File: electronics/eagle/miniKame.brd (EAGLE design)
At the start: 37.8 x 41.9 mm, 17 parts

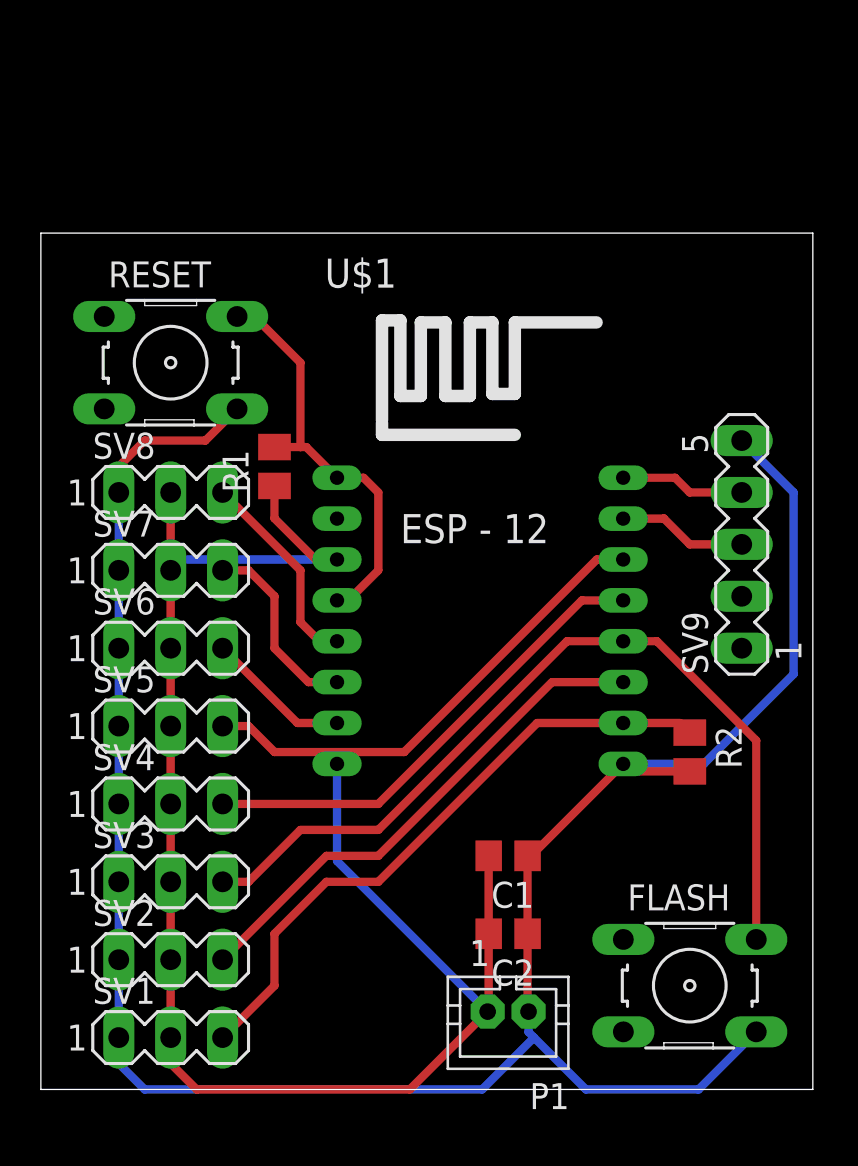
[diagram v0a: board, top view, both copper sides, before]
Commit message: Update pcb
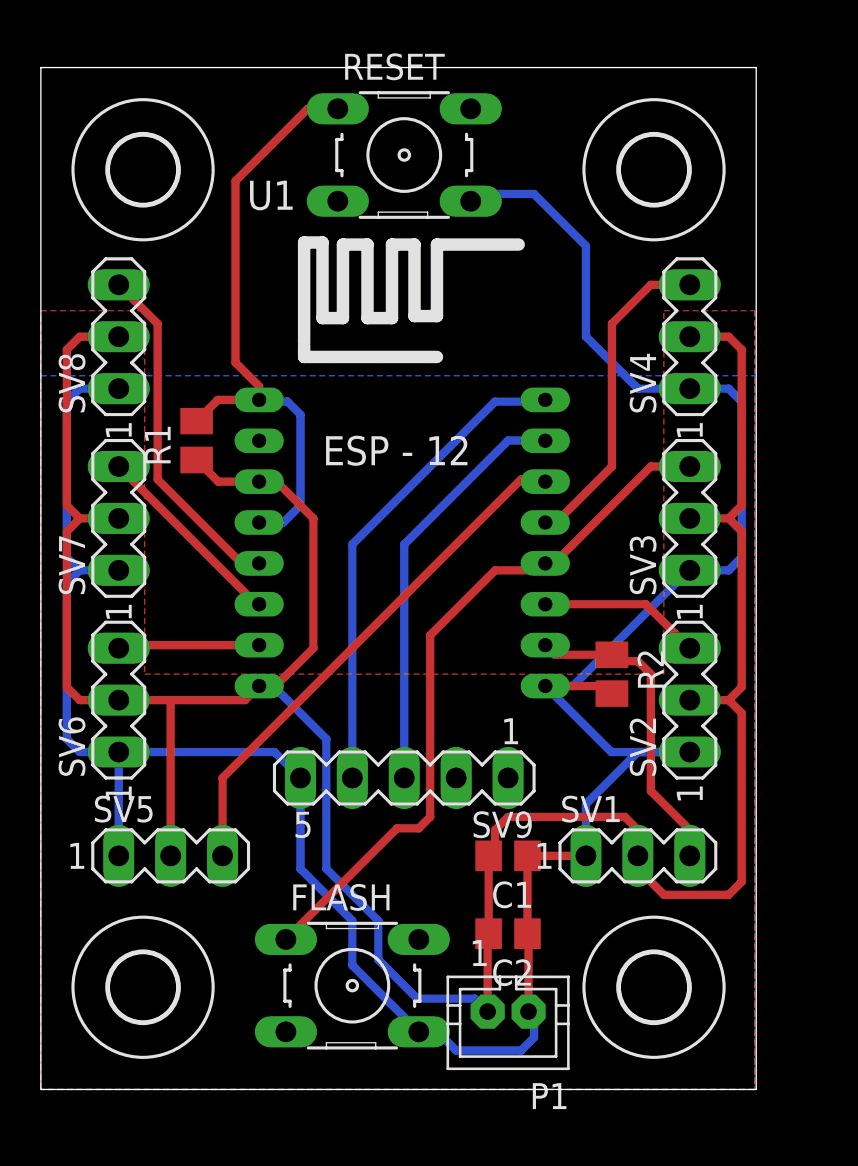
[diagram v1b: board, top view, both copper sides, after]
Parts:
- removed U$1: ESP12, esp8266modules:ESP12
- added H1, H2, H3, H4: MOUNT-HOLE3.3, holes:3,3
- added U1: ESP12, esp8266modules:ESP12
- C1: value (none) -> 100n
- C2: value (none) -> 100u
- moved SV4 34.2 mm to (31.8, 36.8), turned to 90 degrees
- moved SV3 31.0 mm to (31.8, 27.9), turned to 90 degrees
- moved SV2 28.4 mm to (31.8, 19.1), turned to 90 degrees
- moved SV1 24.5 mm to (29.2, 11.4)
- moved SV9 20.1 mm to (17.8, 15.2), turned to 180 degrees
- moved FLASH 16.5 mm to (15.2, 5.08)
- moved RESET 15.3 mm to (17.8, 45.7)
- moved SV8 8.03 mm to (3.81, 36.8), turned to 90 degrees
- moved SV5 6.35 mm to (6.35, 11.4)
- moved R2 5.39 mm to (27.9, 20.3)
- moved R1 4.02 mm to (7.62, 31.8)
- moved SV7 3.59 mm to (3.81, 27.9), turned to 90 degrees
- moved SV6 3.59 mm to (3.81, 19.1), turned to 90 degrees
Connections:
- removed net N$3: SV9.2
- net +3V3: now also U1.CH_PD, U1.VCC; no longer U$1.CH_PD, U$1.VCC
- net GND: now also U1.GND; no longer U$1.GND
- net N$1: now also U1.TX; no longer U$1.TX
- net N$2: now also U1.RX; no longer U$1.RX
- net N$4: now also RESET.1, U1.GPIO16, U1.RESET; no longer RESET.2, U$1.GPIO16, U$1.RESET
- net S1: now also U1.GPIO15; no longer U$1.GPIO15
- net S2: now also U1.GPIO2; no longer U$1.GPIO2
- net S3: now also FLASH.1, U1.GPIO0; no longer FLASH.2, U$1.GPIO0
- net S4: now also U1.GPIO5; no longer U$1.GPIO5
- net S5: now also U1.GPIO4; no longer U$1.GPIO4
- net S6: now also U1.GPIO13; no longer U$1.GPIO13
- net S7: now also U1.GPIO12; no longer U$1.GPIO12
- net S8: now also U1.GPIO14; no longer U$1.GPIO14
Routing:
- net +3V3: track 82.2 -> 136.7 mm
- net GND: track 112.8 -> 132.6 mm
- net N$1: track 6.10 -> 23.8 mm
- net S2: track 25.2 -> 7.96 mm
- net S1: track 30.9 -> 15.4 mm
- net N$2: track 6.33 -> 20.4 mm
- net N$4: track 20.6 -> 30.3 mm
- net S3: track 42.7 -> 34.6 mm
- net S4: track 23.7 -> 16.0 mm
- net S8: track 10.1 -> 17.0 mm
- net S5: track 24.0 -> 25.7 mm
- added copper zone on layer 1, net +3V3
- added copper zone on layer 16, net GND
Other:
- board size 37.8 x 41.9 mm -> 35 x 50 mm
